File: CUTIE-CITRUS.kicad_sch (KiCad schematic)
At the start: 5 parts, among them U1 CM5

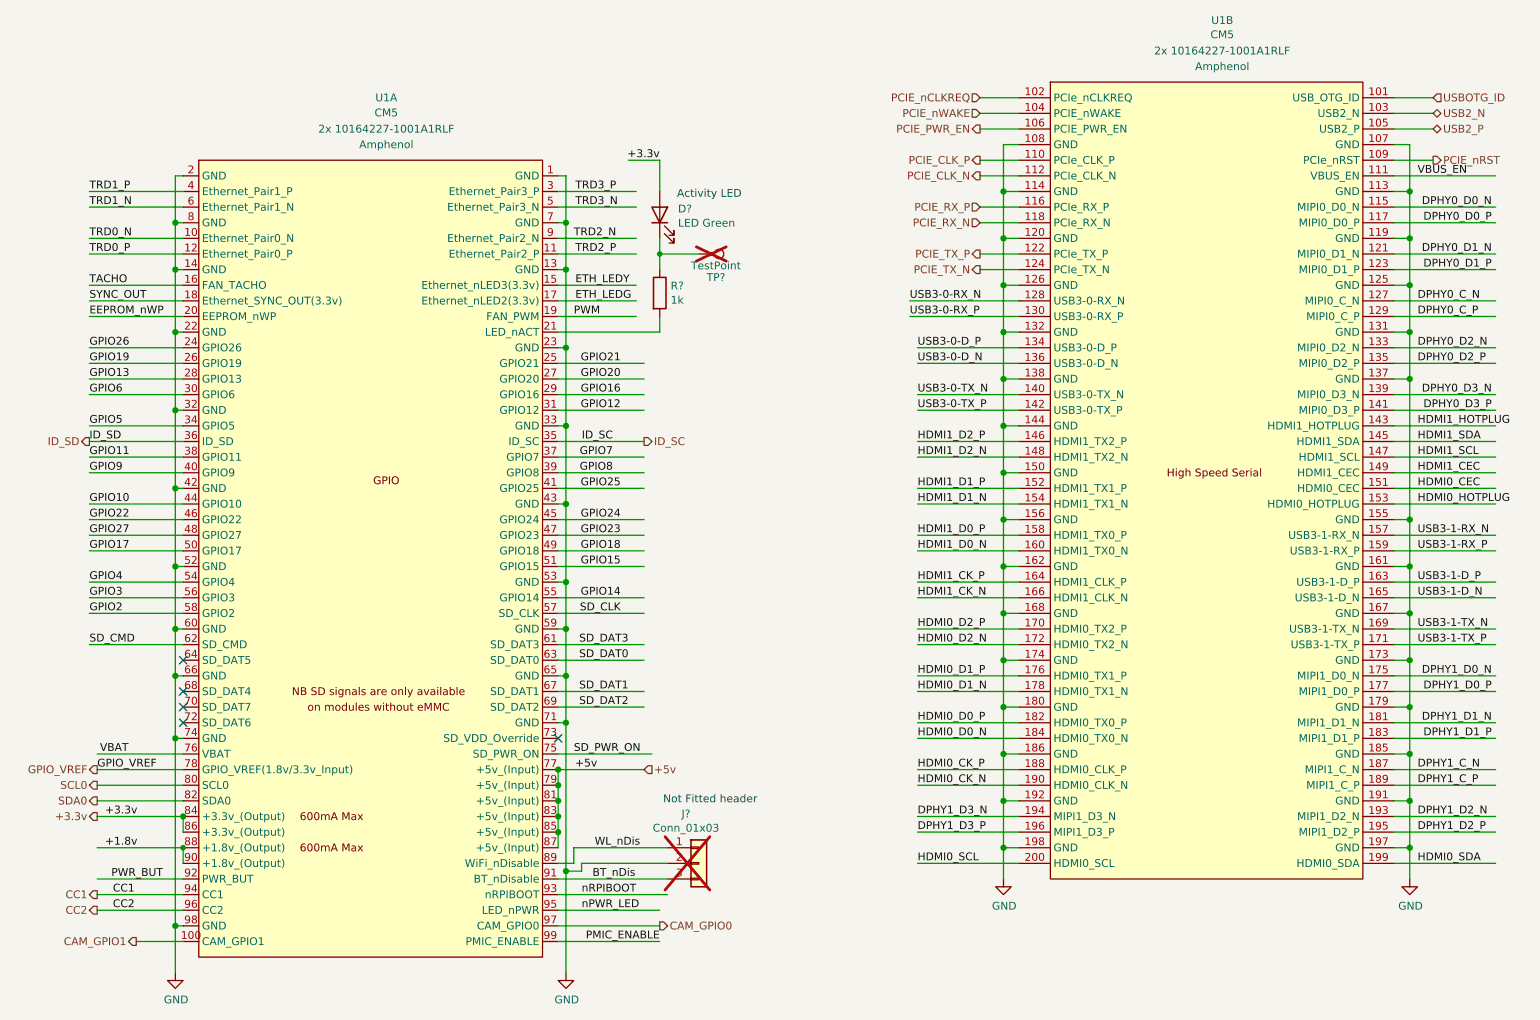
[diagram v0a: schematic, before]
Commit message: saved libs to project, initialized hierarchy
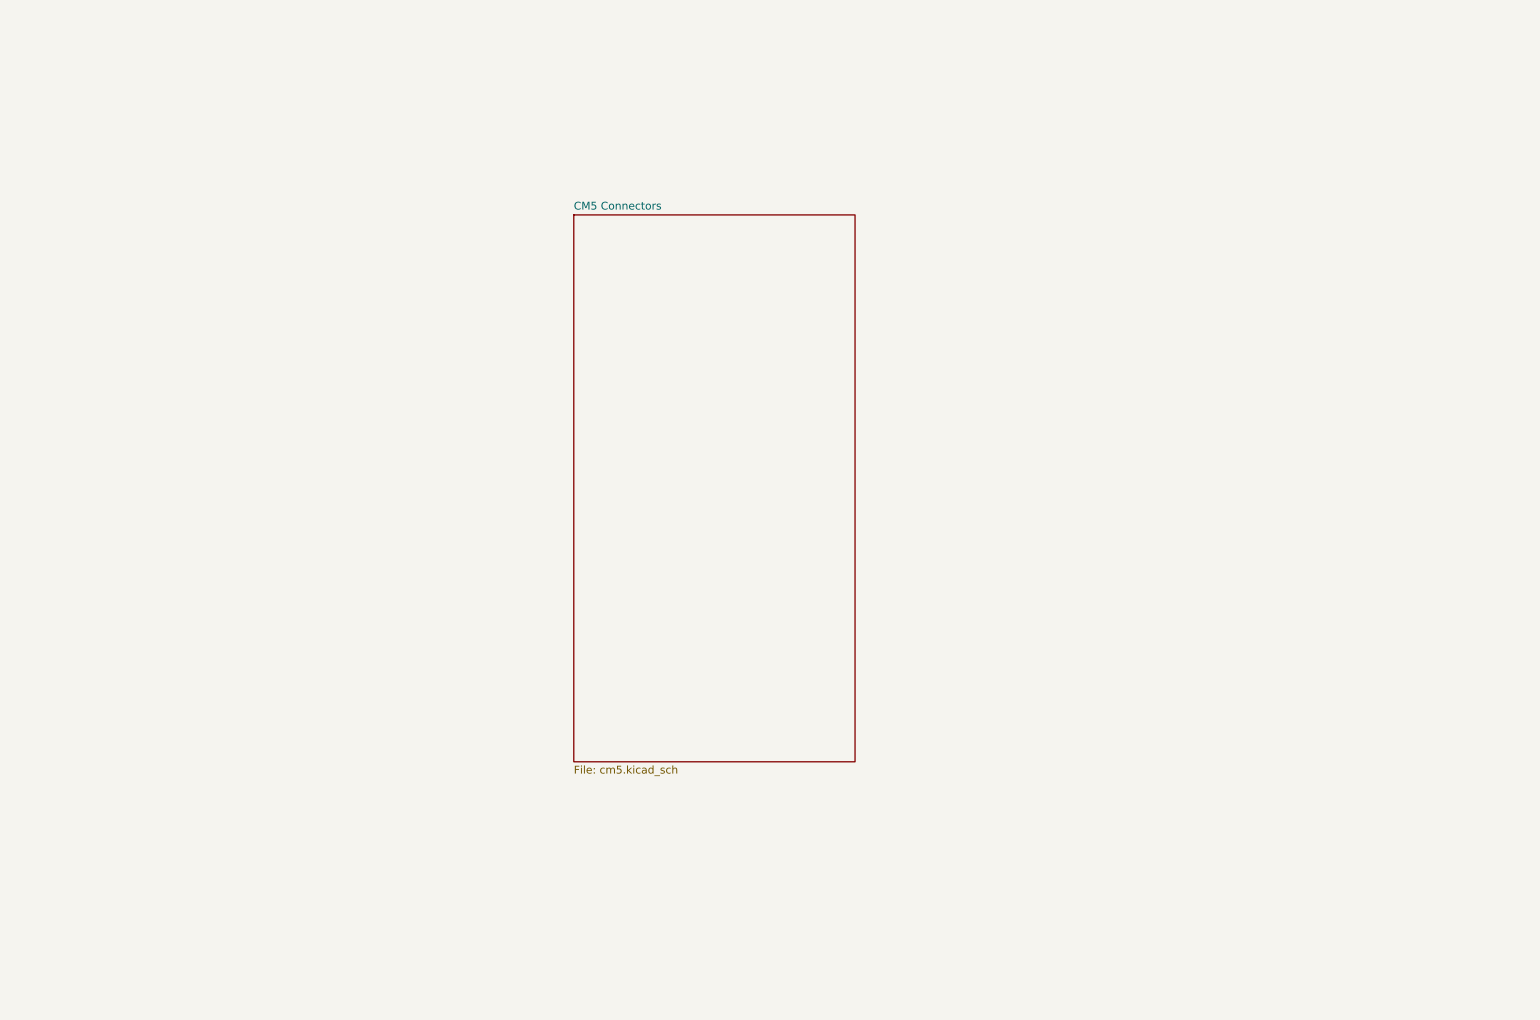
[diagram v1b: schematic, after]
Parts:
- removed D?: LED Green, LED_SMD:LED_0603_1608Metric, symbol Device:LED
- removed J?: Conn_01x03, Connector_PinHeader_2.54mm:PinHeader_1x03_P2.54mm_Vertical, symbol Connector_Generic:Conn_01x03
- removed R?: 1k, Resistor_SMD:R_0402_1005Metric, symbol Device:R
- removed TP?: TestPoint, TestPoint:TestPoint_Pad_2.0x2.0mm, symbol Connector:TestPoint
- removed U1: CM5, CM5IO:Raspberry-Pi-5-Compute-Module, symbol CM5IO:ComputeModule5-CM5
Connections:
- no-connect marks 5 -> 0
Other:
- added sheet CM5 Connectors (cm5.kicad_sch)
- note removed: "Activity LED"
- note removed: "Not Fitted header"
